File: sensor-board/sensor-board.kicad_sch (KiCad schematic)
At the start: 100 parts, among them J1 USB_C_Receptacle_USB2.0_16P, J10 cap3, J11 cap4, J2 Conn_01x06, J3 aux pwr, J4 SWD, J5 water 1, J6 water 2, J7 relay, J8 cap1, J9 cap2, K1 SIL03-1A72-71D, Q1 Si2312, Q2 Si2312, SW1 SW_Push, U1 MLPF-WB55-01E3, U10 EKMB130711, U11 DRV5032, U2 STM32WB55CCUx, U3 MCP1703Ax-300xxTT, U4 SHT40-AD1F-R2, U5 VL53L1CXV0FY1, U6 TLV4082, U7 CLS16D24-44, U8 LIS2DE12TR, U9 FDC2114RGHR, Y1 32MHz, Y2 32.768KHz

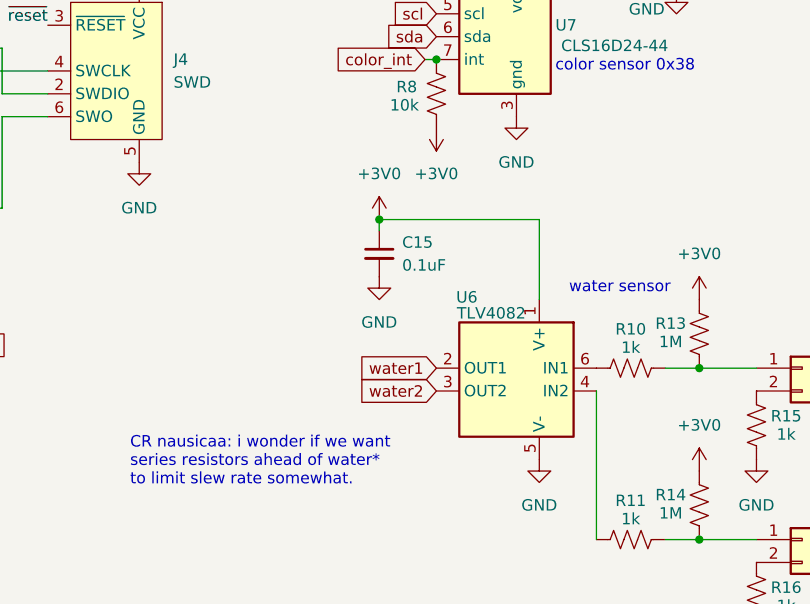
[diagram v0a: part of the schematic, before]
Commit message: DRC-clean
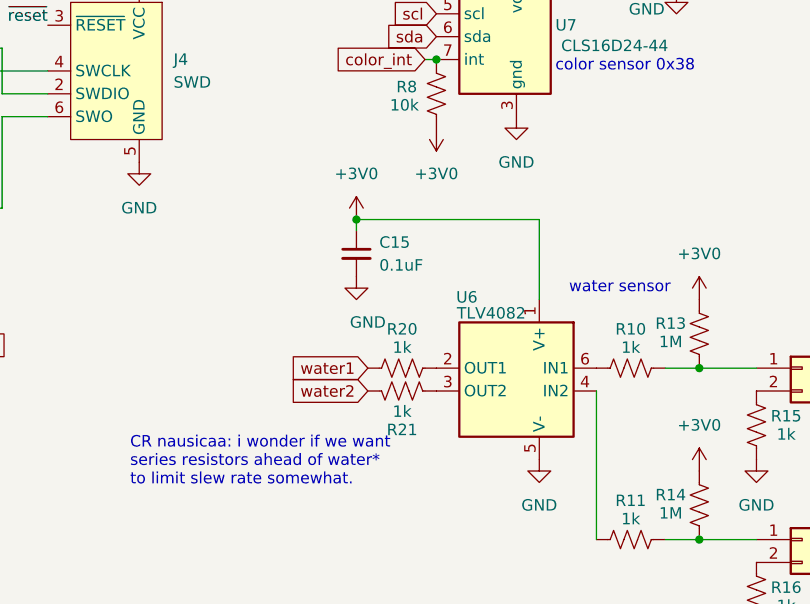
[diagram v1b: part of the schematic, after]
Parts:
- added R20, R21: 1k, Resistor_SMD:R_0402_1005Metric, symbol Device:R_US
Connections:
- net water1: now also R20.1; no longer U6.2 (OUT1)
- net water2: now also R21.1; no longer U6.3 (OUT2)
- new net: R20.2, U6.2 (OUT1)
- new net: R21.2, U6.3 (OUT2)
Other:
- moved on the sheet: C15
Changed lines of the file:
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@@
 	)
 	(junction
-		(at 187.96 101.6)
-		(diameter 0)
-		(color 0 0 0 0)
-	)
-	(junction
 		(at 306.07 66.04)
 		(diameter 0)
@@
 	)
 	(junction
+		(at 185.42 101.6)
+		(diameter 0)
+		(color 0 0 0 0)
+	)
+	(junction
 		(at 77.47 92.71)
 		(diameter 0)
@@
 	(wire
 		(pts
+			(xy 185.42 101.6) (xy 205.74 101.6)
+		)
+		(stroke
+			(width 0)
+			(type default)
+		)
+	)
+	(wire
+		(pts
 			(xy 317.5 66.04) (xy 317.5 67.31)
 		)
@@
 	(wire
 		(pts
-			(xy 205.74 101.6) (xy 187.96 101.6)
-		)
-		(stroke
-			(width 0)
-			(type default)
-		)
-	)
-	(wire
-		(pts
 			(xy 217.17 157.48) (xy 217.17 158.75)
 		)
@@
 	(wire
 		(pts
-			(xy 187.96 101.6) (xy 187.96 102.87)
+			(xy 185.42 101.6) (xy 185.42 102.87)
 		)
 		(stroke
@@
 	(global_label "water1"
 		(shape input)
-		(at 194.31 118.11 180)
+		(at 186.69 118.11 180)
 		(fields_autoplaced yes)
 		(effects
@@
 		)
 		(property "Intersheetrefs" "${INTERSHEET_REFS}"
-			(at 185.0353 118.11 0)
+			(at 177.4153 118.11 0)
 			(hide yes)
 			(show_name no)
@@
 	(global_label "water2"
 		(shape input)
-		(at 194.31 120.65 180)
+		(at 186.69 120.65 180)
 		(fields_autoplaced yes)
 		(effects
@@
 		)
 		(property "Intersheetrefs" "${INTERSHEET_REFS}"
-			(at 185.0353 120.65 0)
+			(at 177.4153 120.65 0)
 			(hide yes)
 			(show_name no)
@@
 	(symbol
 		(lib_id "power:GND")
-		(at 187.96 107.95 0)
+		(at 185.42 107.95 0)
 		(unit 1)
 		(body_style 1)
@@
 		(in_pos_files yes)
 		(dnp no)
-		(fields_autoplaced yes)
 		(property "Reference" "#PWR038"
-			(at 187.96 114.3 0)
+			(at 185.42 114.3 0)
 			(hide yes)
 			(show_name no)
@@
 		)
 		(property "Value" "GND"
-			(at 187.96 113.03 0)
+			(at 186.69 113.03 0)
 			(show_name no)
 			(do_not_autoplace no)
@@
 		)
 		(property "Footprint" ""
-			(at 187.96 107.95 0)
+			(at 185.42 107.95 0)
 			(hide yes)
 			(show_name no)
@@
 		)
 		(property "Datasheet" ""
-			(at 187.96 107.95 0)
+			(at 185.42 107.95 0)
 			(hide yes)
 			(show_name no)
@@
 		)
 		(property "Description" "Power symbol creates a global label with name \"GND\" , ground"
-			(at 187.96 107.95 0)
+			(at 185.42 107.95 0)
 			(hide yes)
 			(show_name no)
@@
 	(symbol
 		(lib_id "Device:C_Small")
-		(at 187.96 105.41 0)
+		(at 185.42 105.41 0)
 		(unit 1)
 		(body_style 1)
@@
 		(fields_autoplaced yes)
 		(property "Reference" "C15"
-			(at 190.5 104.1462 0)
+			(at 187.96 104.1462 0)
 			(show_name no)
 			(do_not_autoplace no)
@@
 		)
 		(property "Value" "0.1uF"
-			(at 190.5 106.6862 0)
+			(at 187.96 106.6862 0)
 			(show_name no)
 			(do_not_autoplace no)
@@
 		)
 		(property "Footprint" "Capacitor_SMD:C_0402_1005Metric"
-			(at 187.96 105.41 0)
+			(at 185.42 105.41 0)
 			(hide yes)
 			(show_name no)
@@
 		)
 		(property "Datasheet" ""
-			(at 187.96 105.41 0)
+			(at 185.42 105.41 0)
 			(hide yes)
 			(show_name no)
@@
 		)
 		(property "Description" "Unpolarized capacitor, small symbol"
-			(at 187.96 105.41 0)
+			(at 185.42 105.41 0)
 			(hide yes)
 			(show_name no)
@@
 	(symbol
 		(lib_id "power:+3V0")
-		(at 187.96 101.6 0)
+		(at 185.42 101.6 0)
 		(unit 1)
 		(body_style 1)
@@
 		(fields_autoplaced yes)
 		(property "Reference" "#PWR037"
-			(at 187.96 105.41 0)
+			(at 185.42 105.41 0)
 			(hide yes)
 			(show_name no)
@@
 		)
 		(property "Value" "+3V0"
-			(at 187.96 96.52 0)
+			(at 185.42 96.52 0)
 			(show_name no)
 			(do_not_autoplace no)
@@
 		)
 		(property "Footprint" ""
-			(at 187.96 101.6 0)
+			(at 185.42 101.6 0)
 			(hide yes)
 			(show_name no)
@@
 		)
 		(property "Datasheet" ""
-			(at 187.96 101.6 0)
+			(at 185.42 101.6 0)
 			(hide yes)
 			(show_name no)
@@
 		)
 		(property "Description" "Power symbol creates a global label with name \"+3V0\""
-			(at 187.96 101.6 0)
+			(at 185.42 101.6 0)
 			(hide yes)
 			(show_name no)
@@
 	)
 	(symbol
+		(lib_id "Device:R_US")
+		(at 190.5 118.11 90)
+		(unit 1)
+		(body_style 1)
+		(exclude_from_sim no)
+		(in_bom yes)
+		(on_board yes)
+		(in_pos_files yes)
+		(dnp no)
+		(property "Reference" "R20"
+			(at 190.5 113.792 90)
+			(show_name no)
+			(do_not_autoplace no)
+			(effects
+				(font
+					(size 1.27 1.27)
+				)
+			)
+		)
+		(property "Value" "1k"
+			(at 190.5 115.824 90)
+			(show_name no)
+			(do_not_autoplace no)
+			(effects
+				(font
+					(size 1.27 1.27)
+				)
+			)
+		)
+		(property "Footprint" "Resistor_SMD:R_0402_1005Metric"
+			(at 190.754 117.094 90)
+			(hide yes)
+			(show_name no)
+			(do_not_autoplace no)
+			(effects
+				(font
+					(size 1.27 1.27)
+				)
+			)
+		)
+		(property "Datasheet" ""
+			(at 190.5 118.11 0)
+			(hide yes)
+			(show_name no)
+			(do_not_autoplace no)
+			(effects
+				(font
+					(size 1.27 1.27)
+				)
+			)
+		)
+		(property "Description" "Resistor, US symbol"
+			(at 190.5 118.11 0)
+			(hide yes)
+			(show_name no)
+			(do_not_autoplace no)
+			(effects
+				(font
+					(size 1.27 1.27)
+				)
+			)
+		)
+		(pin "2"
+		)
+		(pin "1"
+		)
+		(instances
+			(project "sensor-board"
+				(path "/51c2f14d-61ea-40ae-9b85-8b2a49be52ac"
+					(reference "R20")
+					(unit 1)
+				)
+			)
+		)
+	)
+	(symbol
 		(lib_id "vendor:Antenna_InvertedF")
 		(at 20.32 90.17 0)
@@
 					(unit 1)
 				)
+			)
+		)
+	)
+	(symbol
+		(lib_id "Device:R_US")
+		(at 190.5 120.65 90)
+		(mirror x)
+		(unit 1)
+		(body_style 1)
+		(exclude_from_sim no)
+		(in_bom yes)
+		(on_board yes)
+		(in_pos_files yes)
+		(dnp no)
+		(property "Reference" "R21"
+			(at 190.5 124.968 90)
+			(show_name no)
+			(do_not_autoplace no)
+			(effects
+				(font
+					(size 1.27 1.27)
+				)
+			)
+		)
+		(property "Value" "1k"
+			(at 190.5 122.936 90)
+			(show_name no)
+			(do_not_autoplace no)
+			(effects
+				(font
+					(size 1.27 1.27)
+				)
+			)
+		)
+		(property "Footprint" "Resistor_SMD:R_0402_1005Metric"
+			(at 190.754 121.666 90)
+			(hide yes)
+			(show_name no)
+			(do_not_autoplace no)
+			(effects
+				(font
+					(size 1.27 1.27)
+				)
+			)
+		)
+		(property "Datasheet" ""
+			(at 190.5 120.65 0)
+			(hide yes)
+			(show_name no)
+			(do_not_autoplace no)
+			(effects
+				(font
+					(size 1.27 1.27)
+				)
+			)
+		)
+		(property "Description" "Resistor, US symbol"
+			(at 190.5 120.65 0)
+			(hide yes)
+			(show_name no)
+			(do_not_autoplace no)
+			(effects
+				(font
+					(size 1.27 1.27)
+				)
+			)
+		)
+		(pin "2"
+		)
+		(pin "1"
+		)
+		(instances
+			(project "sensor-board"
+				(path "/51c2f14d-61ea-40ae-9b85-8b2a49be52ac"
+					(reference "R21")
+					(unit 1)
+				)
